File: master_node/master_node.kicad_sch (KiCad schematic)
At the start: 29 parts, among them J1 X_Stepper, J10 A1_Encoder, J11 A2_Encoder, J12 R_Encoder, J13 XT60-in, J14 X_Power, J15 Y _Power, J16 Z_Power, J17 A1_Power, J18 A2_Power, J19 R_Power, J2 Y_Stepper, J3 Z_Stepper, J4 A1_Stepper, J5 A2_Stepper, J6 R_Stepper, J7 Y_Encoder, J8 X_Encoder, J9 Z_Encoder, SW1 SW_SPDT, U1 NUCLEO-F446RE, U2 UA78M33CDCYR, U3 UA78M05IDCYR

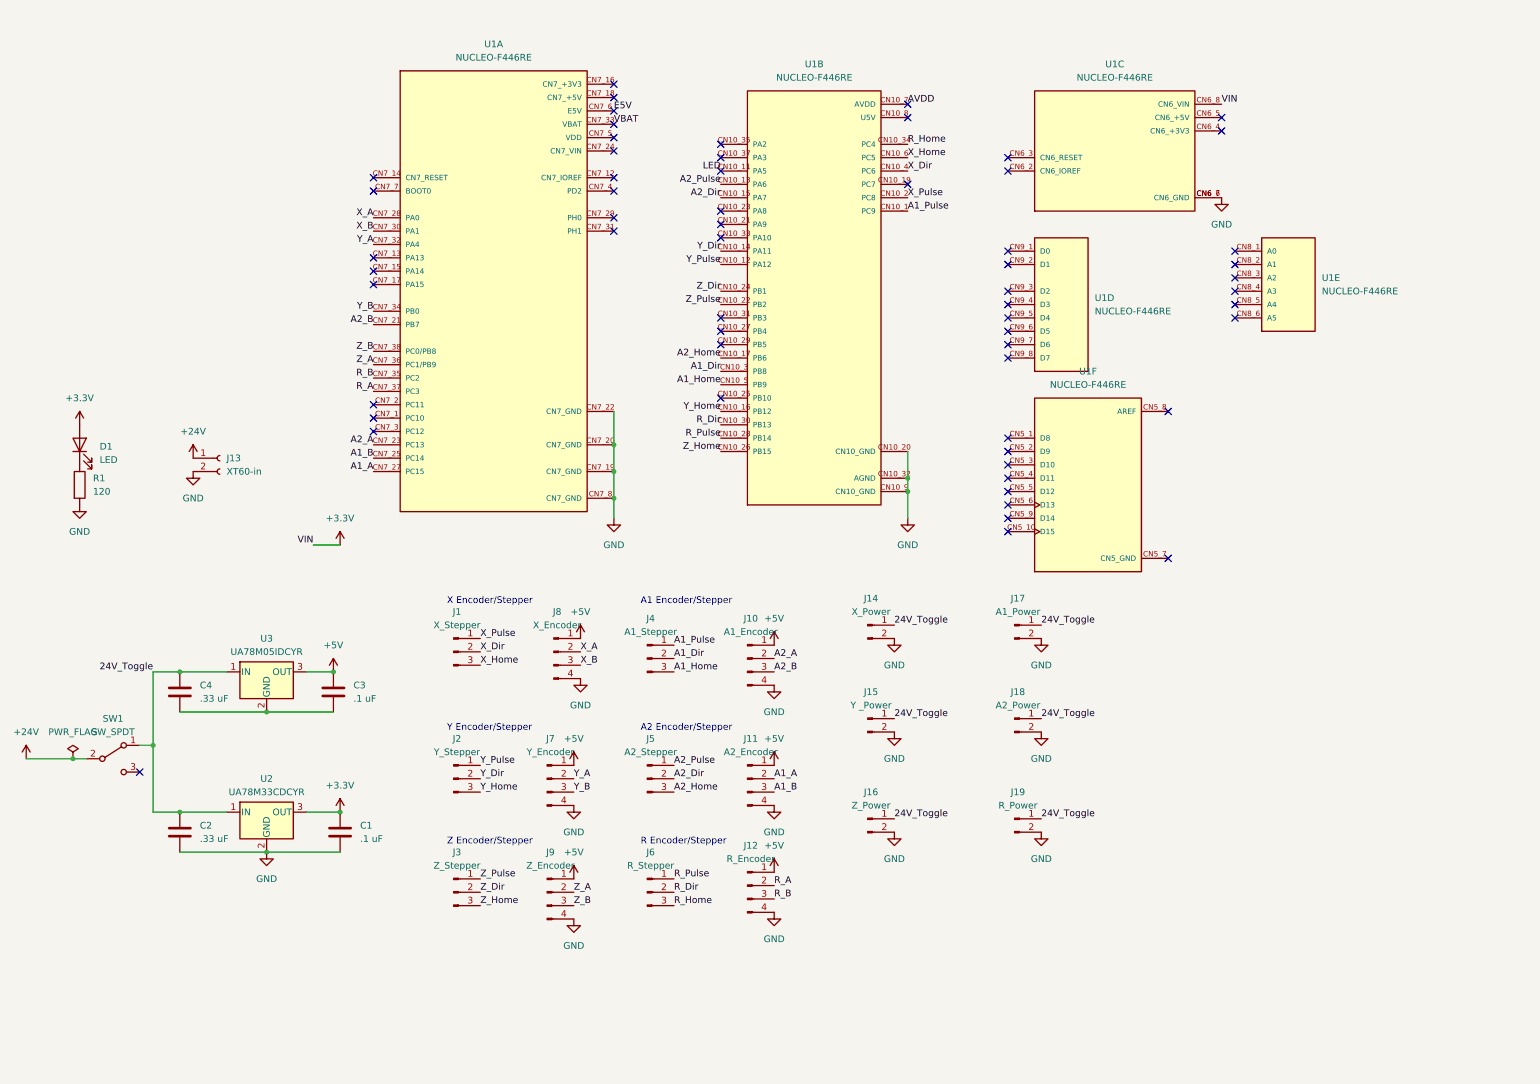
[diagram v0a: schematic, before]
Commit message: too late, I am done
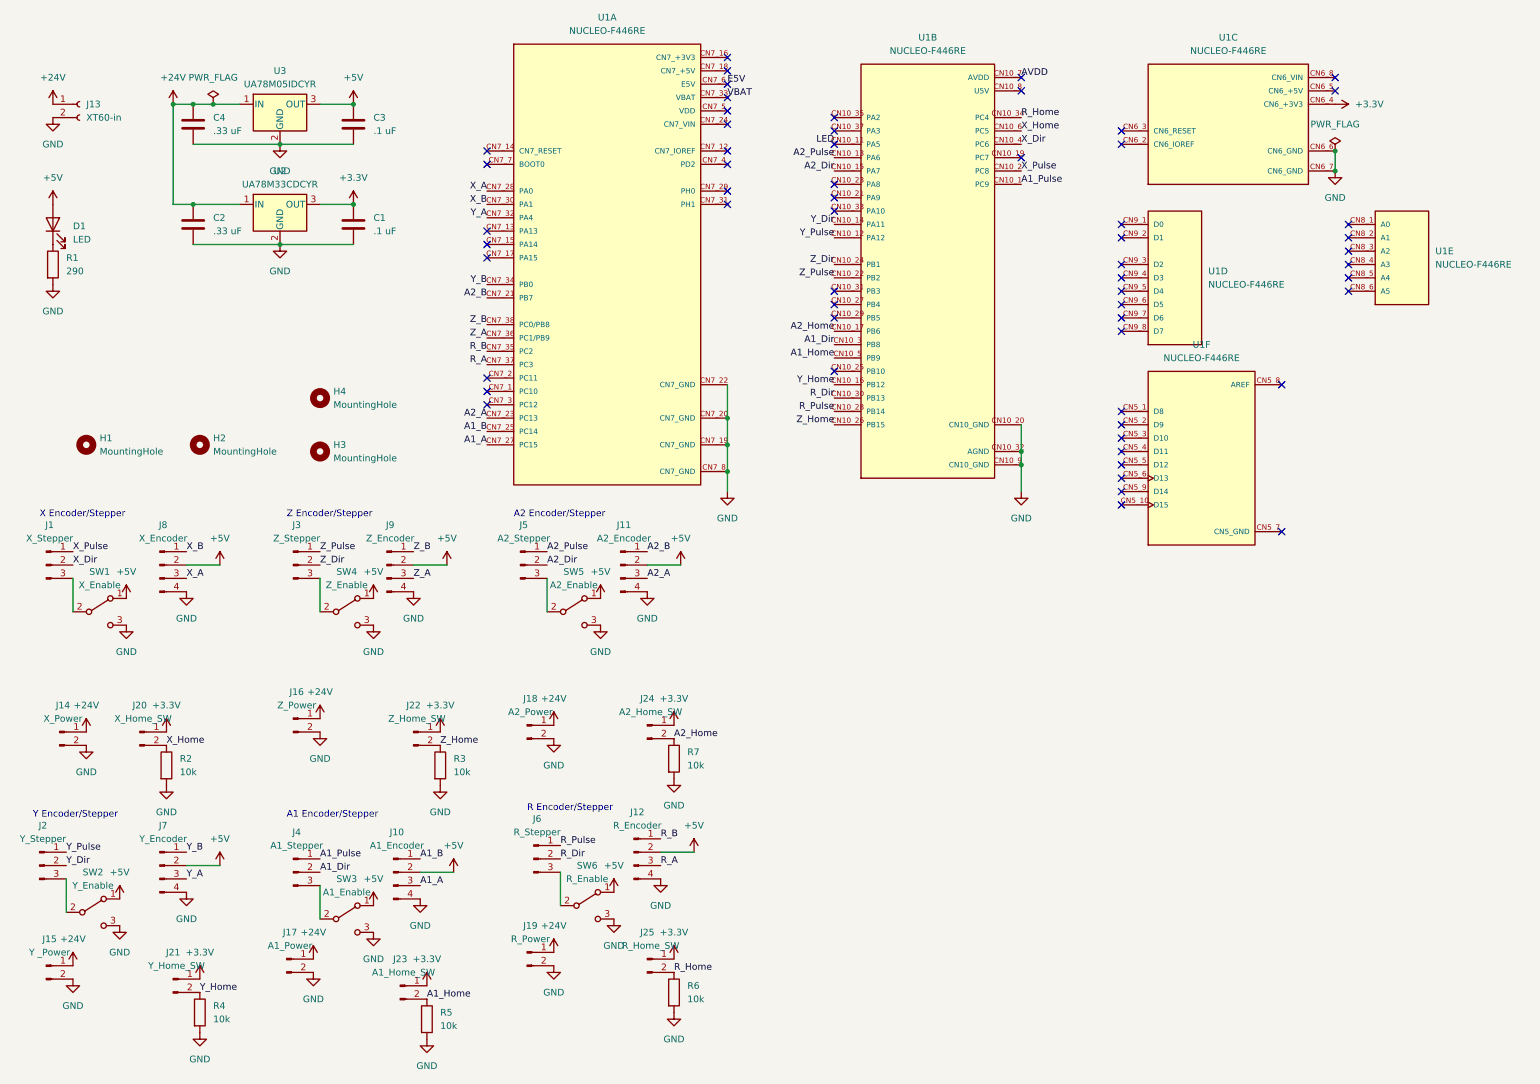
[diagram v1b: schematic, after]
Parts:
- added H1, H2, H3, H4: MountingHole, MountingHole:MountingHole_5.3mm_M5_DIN965, symbol Mechanical:MountingHole
- added J20: X_Home_SW, Connector_PinHeader_2.54mm:PinHeader_1x02_P2.54mm_Vertical, symbol Connector:Conn_01x02_Pin
- added J21: Y_Home_SW, Connector_PinHeader_2.54mm:PinHeader_1x02_P2.54mm_Vertical, symbol Connector:Conn_01x02_Pin
- added J22: Z_Home_SW, Connector_PinHeader_2.54mm:PinHeader_1x02_P2.54mm_Vertical, symbol Connector:Conn_01x02_Pin
- added J23: A1_Home_SW, Connector_PinHeader_2.54mm:PinHeader_1x02_P2.54mm_Vertical, symbol Connector:Conn_01x02_Pin
- added J24: A2_Home_SW, Connector_PinHeader_2.54mm:PinHeader_1x02_P2.54mm_Vertical, symbol Connector:Conn_01x02_Pin
- added J25: R_Home_SW, Connector_PinHeader_2.54mm:PinHeader_1x02_P2.54mm_Vertical, symbol Connector:Conn_01x02_Pin
- added R2, R3, R4, R5, R6, R7: 10k, Resistor_SMD:R_0805_2012Metric_Pad1.20x1.40mm_HandSolder, symbol Device:R
- added SW2: Y_Enable, Button_Switch_THT:SW_CuK_OS102011MA1QN1_SPDT_Angled, symbol Switch:SW_SPDT
- added SW3: A1_Enable, Button_Switch_THT:SW_CuK_OS102011MA1QN1_SPDT_Angled, symbol Switch:SW_SPDT
- added SW4: Z_Enable, Button_Switch_THT:SW_CuK_OS102011MA1QN1_SPDT_Angled, symbol Switch:SW_SPDT
- added SW5: A2_Enable, Button_Switch_THT:SW_CuK_OS102011MA1QN1_SPDT_Angled, symbol Switch:SW_SPDT
- added SW6: R_Enable, Button_Switch_THT:SW_CuK_OS102011MA1QN1_SPDT_Angled, symbol Switch:SW_SPDT
- R1: value 120 -> 290
- SW1: value SW_SPDT -> X_Enable
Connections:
- net +24V: now also C2.2, C4.2, J14.1 (Pin_1), J15.1 (Pin_1), J16.1 (Pin_1), J17.1 (Pin_1), J18.1 (Pin_1), J19.1 (Pin_1), U2.1 (IN), U3.1 (IN); no longer SW1.2 (B)
- net +3.3V: now also U1.CN6_4 (CN6_+3V3), J20.1 (Pin_1), J21.1 (Pin_1), J22.1 (Pin_1), J23.1 (Pin_1), J24.1 (Pin_1), J25.1 (Pin_1); no longer D1.2 (A), U1.CN6_8 (CN6_VIN)
- net +5V: now also D1.2 (A), J10.2 (Pin_2), J11.2 (Pin_2), J12.2 (Pin_2), J7.2 (Pin_2), J8.2 (Pin_2), J9.2 (Pin_2), SW1.1 (A), SW2.1 (A), SW3.1 (A), SW4.1 (A), SW5.1 (A), SW6.1 (A); no longer J10.1 (Pin_1), J11.1 (Pin_1), J12.1 (Pin_1), J7.1 (Pin_1), J8.1 (Pin_1), J9.1 (Pin_1)
- net A1_A: now also J10.3 (Pin_3); no longer J11.2 (Pin_2)
- net A1_B: now also J10.1 (Pin_1); no longer J11.3 (Pin_3)
- net A1_Home: now also J23.2 (Pin_2), R5.1; no longer J4.3 (Pin_3)
- net A2_A: now also J11.3 (Pin_3); no longer J10.2 (Pin_2)
- net A2_B: now also J11.1 (Pin_1); no longer J10.3 (Pin_3)
- net A2_Home: now also J24.2 (Pin_2), R7.1; no longer J5.3 (Pin_3)
- net GND: now also C3.2, C4.1, SW1.3 (C), U3.2 (GND), R2.2, R3.2, R4.2, R5.2, R6.2, R7.2, SW2.3 (C), SW3.3 (C), SW4.3 (C), SW5.3 (C), SW6.3 (C)
- net R_A: now also J12.3 (Pin_3); no longer J12.2 (Pin_2)
- net R_B: now also J12.1 (Pin_1); no longer J12.3 (Pin_3)
- net R_Home: now also J25.2 (Pin_2), R6.1; no longer J6.3 (Pin_3)
- net X_A: now also J8.3 (Pin_3); no longer J8.2 (Pin_2)
- net X_B: now also J8.1 (Pin_1); no longer J8.3 (Pin_3)
- net X_Home: now also J20.2 (Pin_2), R2.1; no longer J1.3 (Pin_3)
- net Y_A: now also J7.3 (Pin_3); no longer J7.2 (Pin_2)
- net Y_B: now also J7.1 (Pin_1); no longer J7.3 (Pin_3)
- net Y_Home: now also J21.2 (Pin_2), R4.1; no longer J2.3 (Pin_3)
- net Z_A: now also J9.3 (Pin_3); no longer J9.2 (Pin_2)
- net Z_B: now also J9.1 (Pin_1); no longer J9.3 (Pin_3)
- net Z_Home: now also J22.2 (Pin_2), R3.1; no longer J3.3 (Pin_3)
- removed net 24V_Toggle: C2.2, C4.2, J14.1 (Pin_1), J15.1 (Pin_1), J16.1 (Pin_1), J17.1 (Pin_1), J18.1 (Pin_1), J19.1 (Pin_1), SW1.1 (A), U2.1 (IN), U3.1 (IN)
- new net: J1.3 (Pin_3), SW1.2 (B)
- new net: J5.3 (Pin_3), SW5.2 (B)
- new net: J2.3 (Pin_3), SW2.2 (B)
- new net: J3.3 (Pin_3), SW4.2 (B)
- new net: J4.3 (Pin_3), SW3.2 (B)
- new net: J6.3 (Pin_3), SW6.2 (B)
- no-connect marks 60 -> 59
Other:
- moved on the sheet: C1, C2, C3, C4, D1, J1, J10, J11, J12, J13, J14, J15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
